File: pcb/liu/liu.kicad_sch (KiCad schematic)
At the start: 14 parts

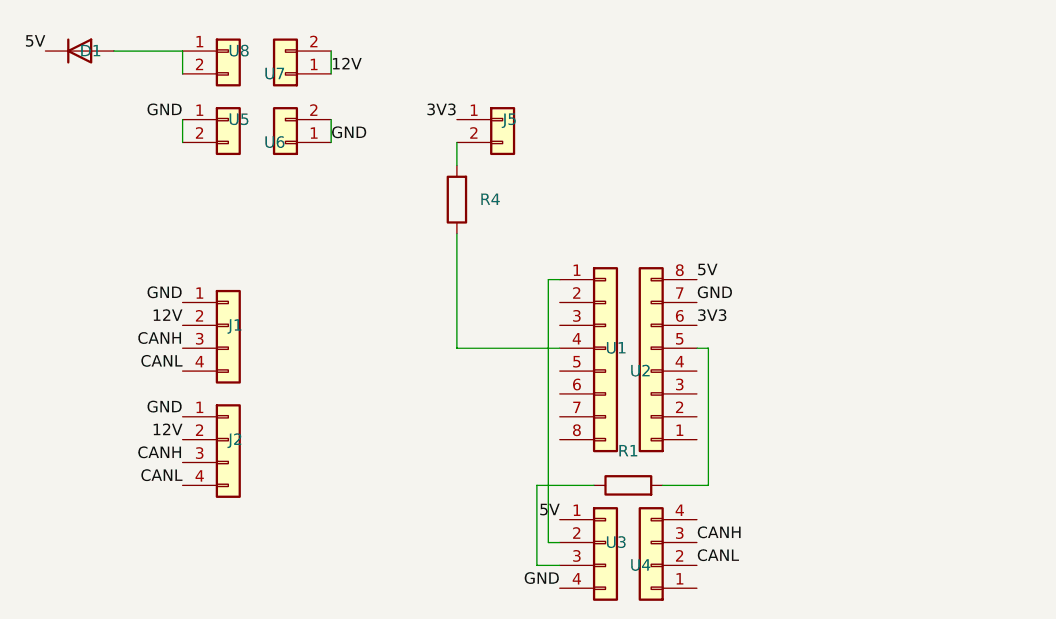
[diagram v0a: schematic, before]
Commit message: liu
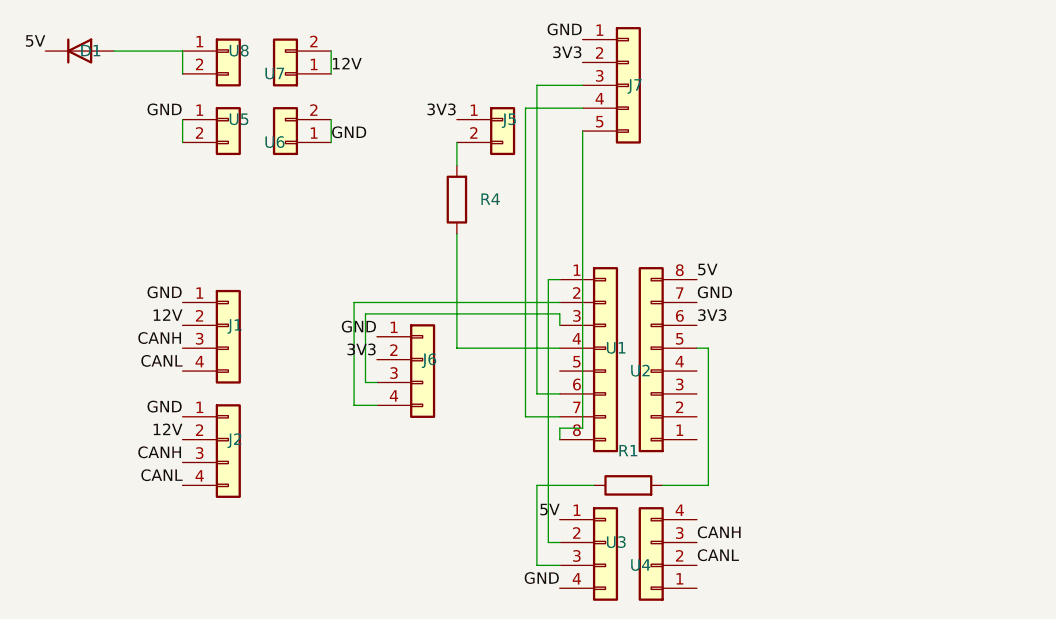
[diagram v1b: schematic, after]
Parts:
- added J6: (no value), Connector_PinSocket_2.54mm:PinSocket_1x04_P2.54mm_Vertical, symbol Connector_Generic:Conn_01x04
- added J7: (no value), Connector_PinSocket_2.54mm:PinSocket_1x05_P2.54mm_Vertical, symbol Connector_Generic:Conn_01x05
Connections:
- net 3V3: now also J6.2 (Pin_2), J7.2 (Pin_2)
- net GND: now also J6.1 (Pin_1), J7.1 (Pin_1)
- net at U1.2 (Pin_2): now also J6.4 (Pin_4)
- net at U1.3 (Pin_3): now also J6.3 (Pin_3)
- net at U1.6 (Pin_6): now also J7.3 (Pin_3)
- net at U1.7 (Pin_7): now also J7.4 (Pin_4)
- net at U1.8 (Pin_8): now also J7.5 (Pin_5)

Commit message: pcb
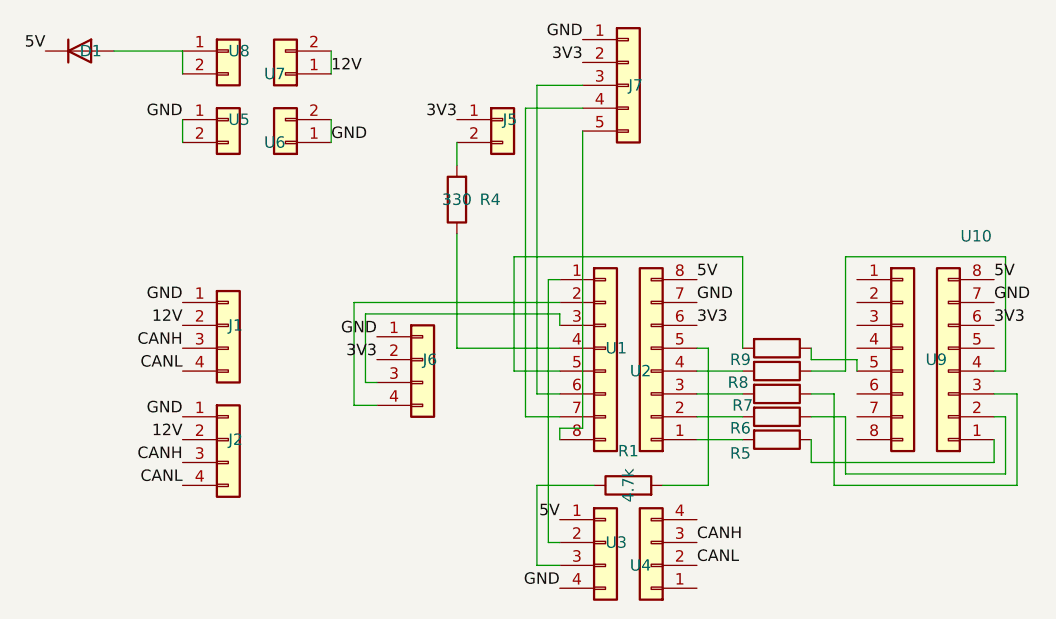
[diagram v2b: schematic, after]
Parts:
- added R5, R6, R7, R8, R9: 1k, Resistor_SMD:R_0603_1608Metric, symbol Device:R
- added U10, U9: (no value), Connector_PinSocket_2.54mm:PinSocket_1x08_P2.54mm_Vertical, symbol Connector_Generic:Conn_01x08
- R1: value (none) -> 4.7k
- R4: value (none) -> 330
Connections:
- net 3V3: now also U10.6 (Pin_6)
- net 5V: now also U10.8 (Pin_8)
- net GND: now also U10.7 (Pin_7)
- net at U2.1 (Pin_1): now also R5.2
- net at U2.2 (Pin_2): now also R6.2
- net at U2.3 (Pin_3): now also R7.2
- net at U2.4 (Pin_4): now also R8.2
- net at U1.5 (Pin_5): now also R9.2
- new net: R5.1, U10.1 (Pin_1)
- new net: R6.1, U10.2 (Pin_2)
- new net: R7.1, U10.3 (Pin_3)
- new net: R8.1, U10.4 (Pin_4)
- new net: R9.1, U9.5 (Pin_5)
